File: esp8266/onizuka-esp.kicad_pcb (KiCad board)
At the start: 2 copper layers, 49 x 19 mm, 7 parts, among them U1 ESP-01, U2 ESP-12E

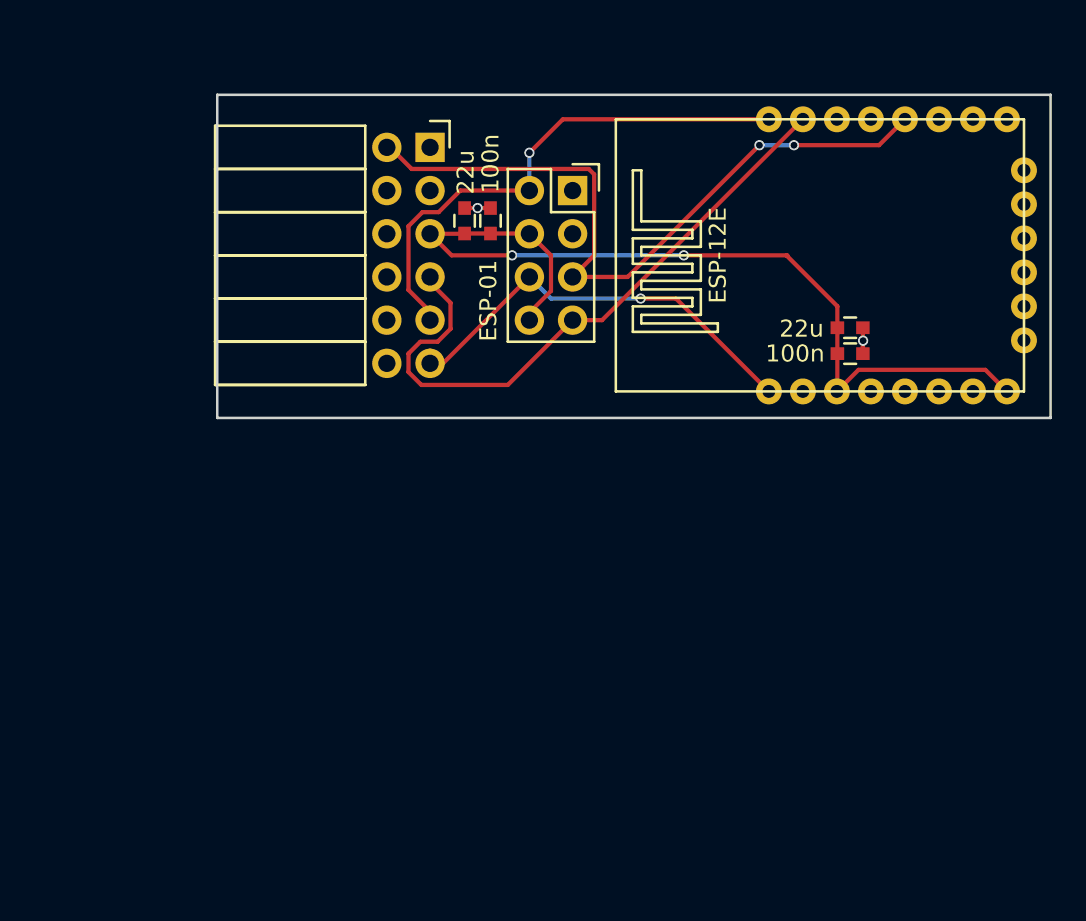
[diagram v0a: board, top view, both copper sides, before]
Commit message: Many faffing, new ESP stuff.
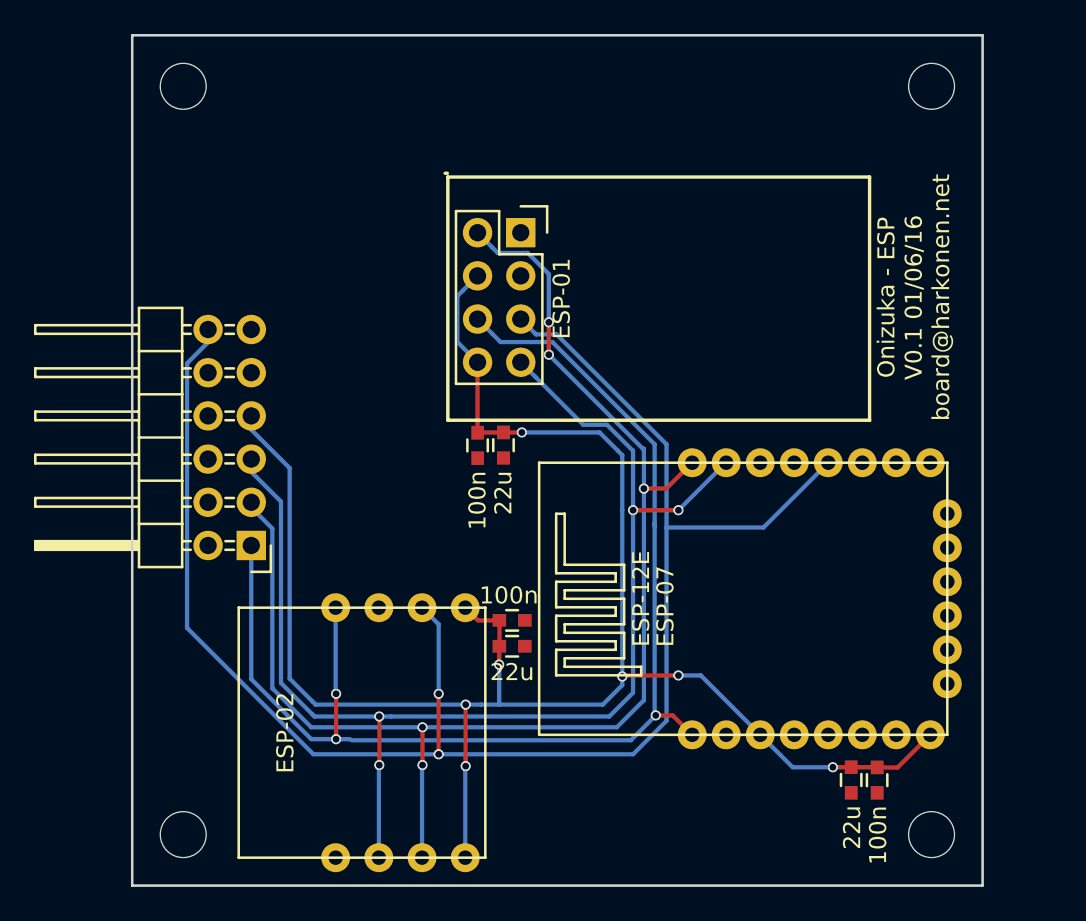
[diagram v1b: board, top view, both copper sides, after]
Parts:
- removed C5: FTDI_CONN, Socket_Strips:Socket_Strip_Angled_2x06
- added C6: 100n, Capacitors_SMD:C_0603, F.Cu at (37.3, 49.4)
- added C7: 22u, Capacitors_SMD:C_0603, F.Cu at (37.3, 50.9)
- added P1: FTDI_CONN, Pin_Headers:Pin_Header_Angled_2x06, F.Cu at (22.0, 45.0)
- added REF**: MountingHole_2.7mm_M2.5, Mounting_Holes:MountingHole_2.7mm_M2.5, F.Cu at (18.0, 18.0)
- added REF**: MountingHole_2.7mm_M2.5, Mounting_Holes:MountingHole_2.7mm_M2.5, F.Cu at (18.0, 62.0)
- added REF**: MountingHole_2.7mm_M2.5, Mounting_Holes:MountingHole_2.7mm_M2.5, F.Cu at (62.0, 62.0)
- added REF**: MountingHole_2.7mm_M2.5, Mounting_Holes:MountingHole_2.7mm_M2.5, F.Cu at (62.0, 18.0)
- added U3: ESP-02, ESP:ESP-02-Program, F.Cu at (28.5, 56.0)
- U2: footprint esp:ESP-12E -> ESP:ESP-12E-Program
- moved C3 26.6 mm to (57.3, 58.8), turned to 270 degrees
- moved C4 25.1 mm to (58.8, 58.8), turned to 270 degrees
- moved U2 20.7 mm to (50.9, 48.1)
- moved C2 13.4 mm to (36.8, 39.1), turned to 270 degrees
- moved C1 13.2 mm to (35.3, 39.1), turned to 270 degrees
- moved U1 3.93 mm to (37.8, 26.6)
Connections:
- U1 pad 3: (no net) -> Net-(U1-Pad3)
- U2 pad 10: (no net) -> Net-(U2-Pad10)
- U2 pad 11: (no net) -> Net-(U2-Pad11)
- U2 pad 12: (no net) -> Net-(U2-Pad12)
- U2 pad 13: (no net) -> Net-(U2-Pad13)
- U2 pad 14: (no net) -> Net-(U2-Pad14)
- U2 pad 16: (no net) -> Net-(U2-Pad16)
- U2 pad 17: (no net) -> Net-(U2-Pad17)
- U2 pad 19: (no net) -> Net-(U2-Pad19)
- U2 pad 2: (no net) -> Net-(U2-Pad2)
- U2 pad 20: (no net) -> Net-(U2-Pad20)
- U2 pad 4: (no net) -> Net-(U2-Pad4)
- U2 pad 5: (no net) -> Net-(U2-Pad5)
- U2 pad 6: (no net) -> Net-(U2-Pad6)
- U2 pad 7: (no net) -> Net-(U2-Pad7)
- U2 pad 9: (no net) -> Net-(U2-Pad9)
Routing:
- net /DTR: track 43.3 -> 98.1 mm
- net VCC: track 53.9 -> 107.3 mm, vias 2 -> 7
- net /RTS: track 26.1 -> 73.6 mm, vias 1 -> 3
- net /RXD: track 31.9 -> 78.7 mm, vias 1 -> 5
- net /TXD: track 37.9 -> 73.9 mm, vias 0 -> 4
- net GND: track 3.83 -> 0.00 mm, vias 2 -> 0
- added copper zone on F.Cu, net GND
- removed copper zone on B.Cu, net GND
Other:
- board size 49 x 19 mm -> 50 x 50 mm
- rule pad_to_mask_clearance: 0.2 -> 0
- board text added: "ESP-07"
